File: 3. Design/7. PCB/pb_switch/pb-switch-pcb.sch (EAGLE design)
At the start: 9 parts, among them SW1 B3F-1000

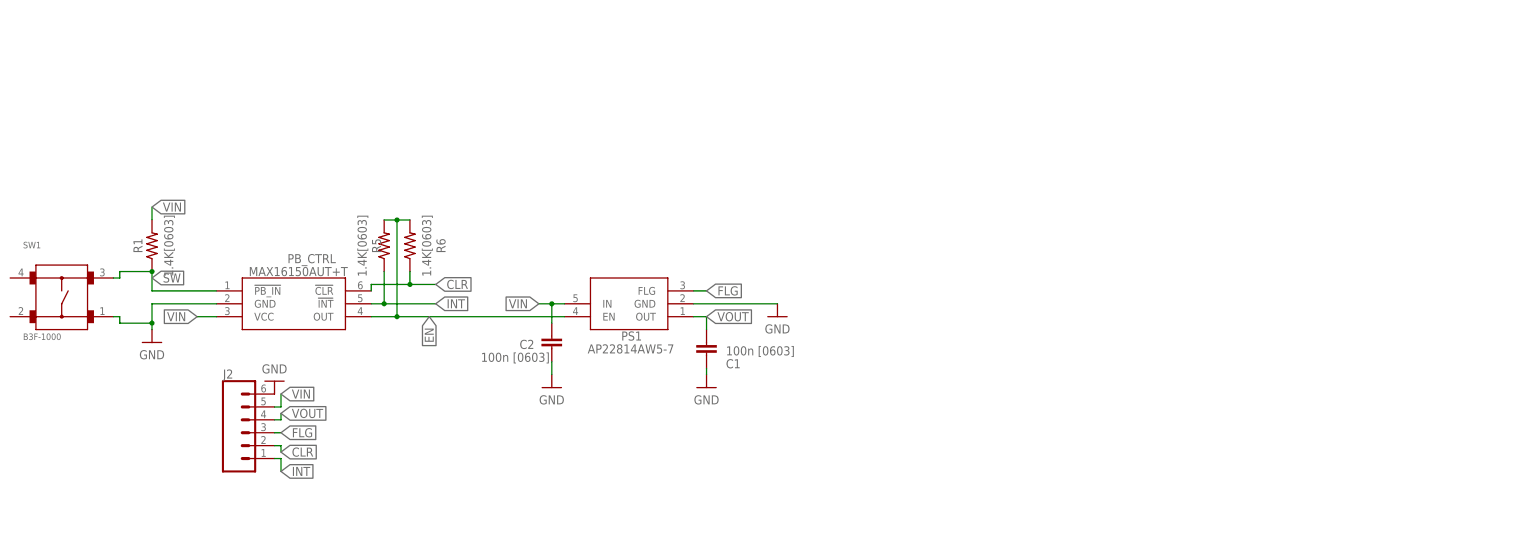
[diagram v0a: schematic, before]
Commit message: ADD|UPDT: Exported new and corrected old 3D models, 2D models and technical drawings of all  PCBs
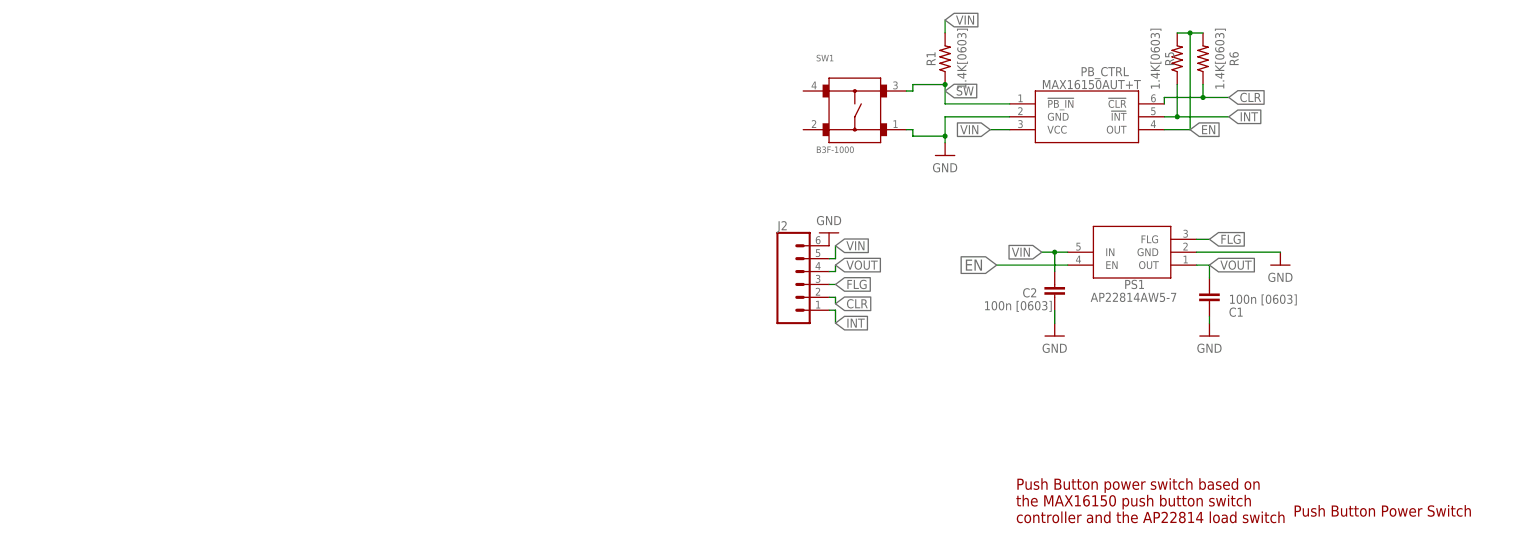
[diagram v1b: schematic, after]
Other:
- note added: "Push Button Power Switch"
- note added: "Push Button power switch based on the MAX16150 push button switch controller and the AP22814 load switch"
- moved on the sheet: C1, C2, J2, PB_CTRL, PS1, R1, R5, R6, SW1
